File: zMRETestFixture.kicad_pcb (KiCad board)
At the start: 2 copper layers, 106.7 x 124.5 mm, 117 parts, among them J1 Conn_01x01, J2 Conn_01x01, J3 Conn_01x01, J4 Conn_01x01, J5 Conn_01x01, J6 Conn_01x01, J7 Conn_02x05_Counter_Clockwise, J8 Conn_01x01_Female, J9 Conn_01x01_Female, SW1 SW_Push, SW2 SW_Push, U1 molex_48pin_MRE

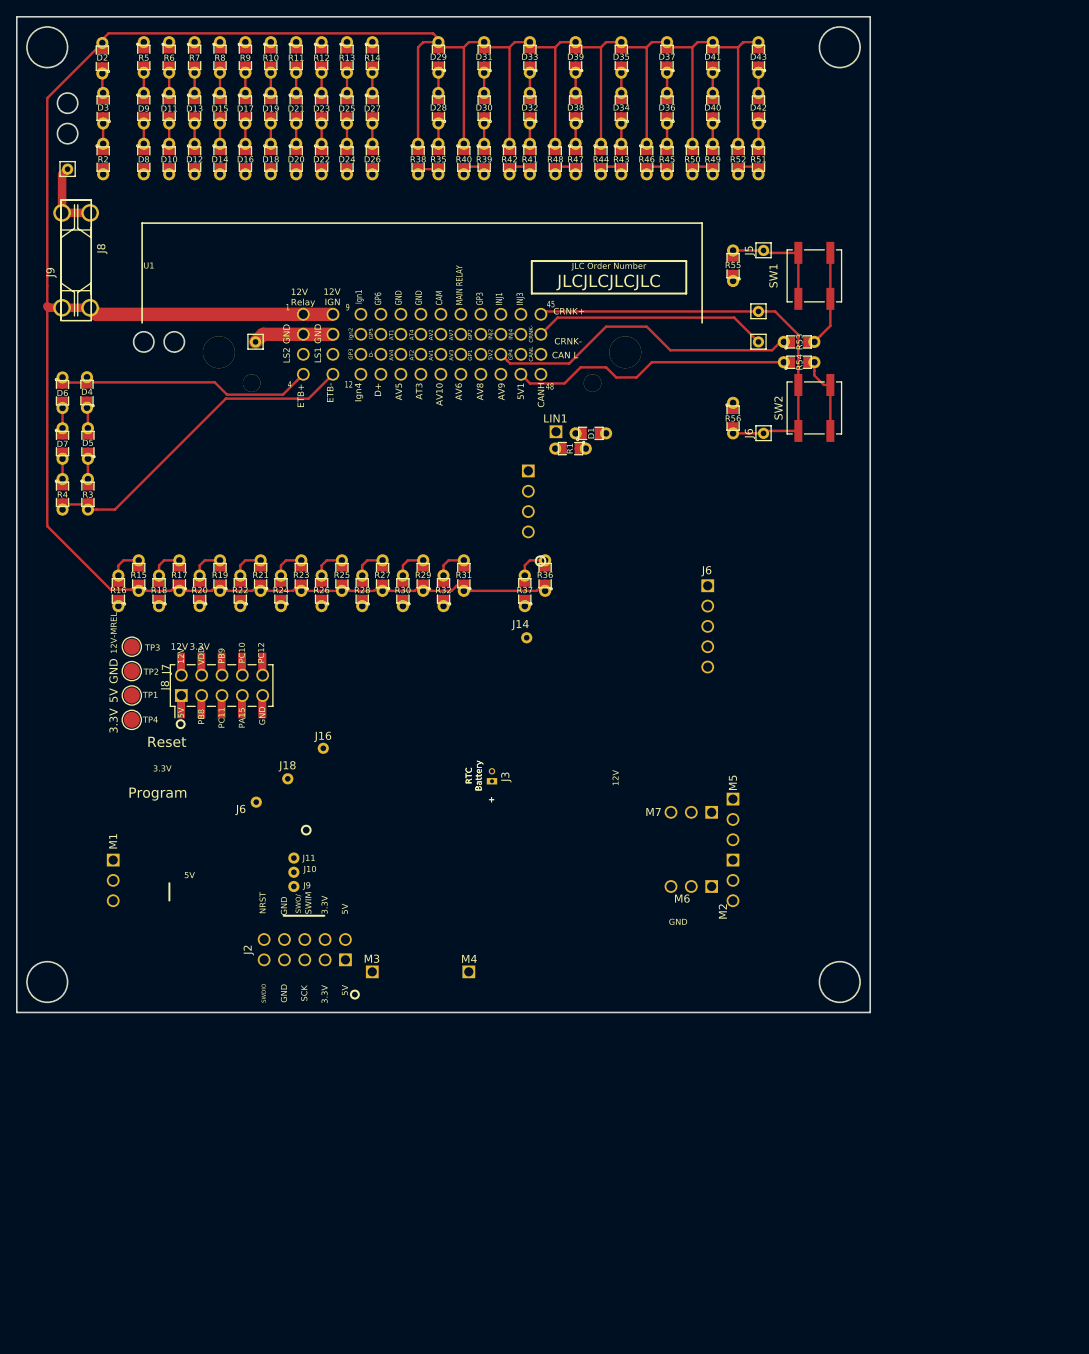
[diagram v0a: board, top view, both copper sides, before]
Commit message: Draft
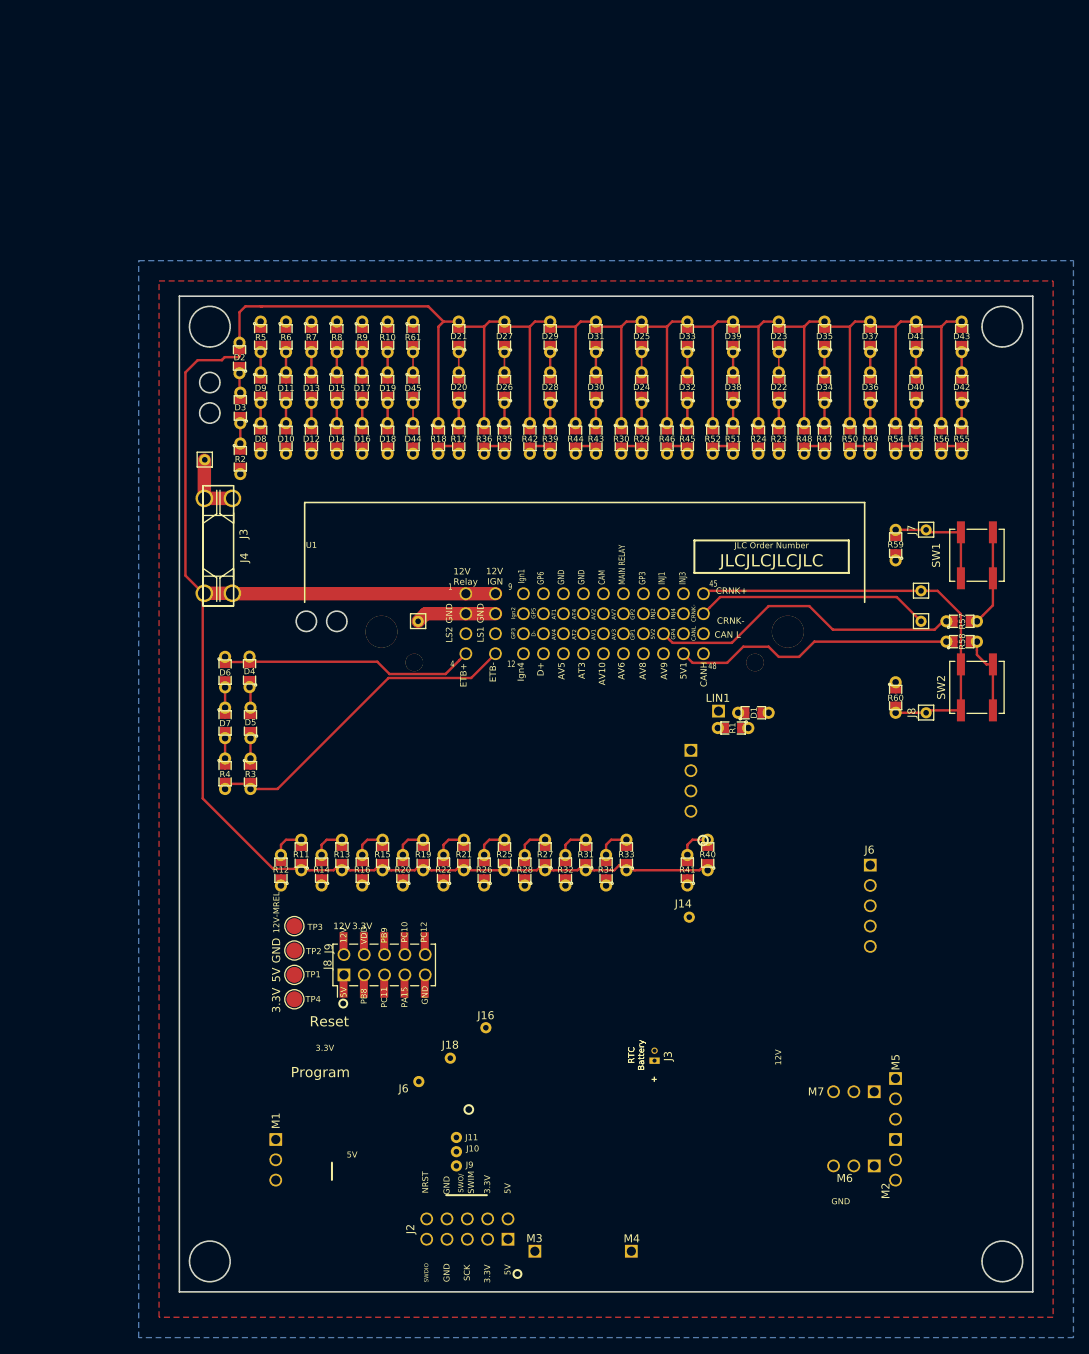
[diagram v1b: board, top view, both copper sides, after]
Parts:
- removed the R11 at (45.1, -2.54)
- removed the R12 at (48.3, -2.54)
- removed the R13 at (51.4, -2.54)
- removed the R14 at (54.6, -2.54)
- removed the R43 at (85.7, 10.2)
- removed the R44 at (83.2, 10.2)
- removed the R45 at (91.4, 10.2)
- removed the R46 at (88.9, 10.2)
- removed the R51 at (102.9, 10.2)
- removed the R52 at (100.3, 10.2)
- added D44: 1N4148WS, rusefi_lib:SM0805_jumper, F.Cu at (59.7, 45.1)
- added D45: GRN, rusefi_lib:SM0805_jumper, F.Cu at (59.7, 38.7)
- added R17: 1k, rusefi_lib:SM0805_jumper, F.Cu at (65.4, 45.1)
- added R18: 5k, rusefi_lib:SM0805_jumper, F.Cu at (62.9, 45.1)
- added R23: 1k, rusefi_lib:SM0805_jumper, F.Cu at (105.4, 45.1)
- added R24: 5k, rusefi_lib:SM0805_jumper, F.Cu at (102.9, 45.1)
- added R29: 1k, rusefi_lib:SM0805_jumper, F.Cu at (88.3, 45.1)
- added R30: 5k, rusefi_lib:SM0805_jumper, F.Cu at (85.7, 45.1)
- added R35: 1k, rusefi_lib:SM0805_jumper, F.Cu at (71.1, 45.1)
- added R36: 5k, rusefi_lib:SM0805_jumper, F.Cu at (68.6, 45.1)
- added R47: 1k, rusefi_lib:SM0805_jumper, F.Cu at (111.1, 45.1)
- added R48: 5k, rusefi_lib:SM0805_jumper, F.Cu at (108.6, 45.1)
- added R53: 1k, rusefi_lib:SM0805_jumper, F.Cu at (122.6, 45.1)
- added R54: 5k, rusefi_lib:SM0805_jumper, F.Cu at (120.0, 45.1)
- added R55: 1k, rusefi_lib:SM0805_jumper, F.Cu at (128.3, 45.1)
- added R56: 5k, rusefi_lib:SM0805_jumper, F.Cu at (125.7, 45.1)
- added R61: 1k, rusefi_lib:SM0805_jumper, F.Cu at (59.7, 32.4)
- D20, D22, D24, D26: value 1N4148WS -> RED
- D21, D23, D25, D27: value BLU -> 1N4148WS
- moved D22 63.9 mm to (105.4, 38.7), turned to 90 degrees
- moved D23 63.9 mm to (105.4, 32.4), turned to 90 degrees
- moved D24 46.6 mm to (88.3, 38.7), turned to 90 degrees
- moved D25 46.6 mm to (88.3, 32.4), turned to 90 degrees
- moved D34 43.2 mm to (111.1, 38.7)
- moved D35 43.2 mm to (111.1, 32.4)
- moved D36 43.2 mm to (116.8, 38.7)
- moved D37 43.2 mm to (116.8, 32.4)
- moved D40 43.2 mm to (122.6, 38.7)
- moved D41 43.2 mm to (122.6, 32.4)
- moved D42 43.2 mm to (128.3, 38.7)
- moved D43 43.2 mm to (128.3, 32.4)
- moved R2 41.2 mm to (38.1, 47.6)
- moved D2 41.2 mm to (38.0, 35.0)
- moved D3 41.2 mm to (38.1, 41.3)
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- renumbered J8 to J3, J9 to J4, J3 to J5, J4 to J6, J5 to J7, J6 to J8, J7 to J9, R15 to R11, R16 to R12, R17 to R13, R18 to R14, R19 to R15, R20 to R16, R21 to R19, R22 to R20, R23 to R21, R24 to R22, R29 to R31, R30 to R32, R31 to R33, R32 to R34, R35 to R39, R36 to R40, R37 to R41, R38 to R42, R39 to R43, R40 to R44, R41 to R45, R42 to R46, R47 to R51, R48 to R52, R53 to R57, R54 to R58, R55 to R59, R56 to R60
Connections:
- D16 pad 2: /GP1 -> /GP6
- D18 pad 2: /GP2 -> /GP5
- D20 pad 2: /GP3 -> Net-(D20-Pad2)
- D21 pad 1: Net-(D21-Pad1) -> Net-(D20-Pad2)
- D21 pad 2: Net-(D20-Pad1) -> /12V_KEY
- D22 pad 2: /GP4 -> Net-(D22-Pad2)
- D23 pad 1: Net-(D23-Pad1) -> Net-(D22-Pad2)
- D23 pad 2: Net-(D22-Pad1) -> /12V_KEY
- D24 pad 2: /GP5 -> Net-(D24-Pad2)
- D25 pad 1: Net-(D25-Pad1) -> Net-(D24-Pad2)
- D25 pad 2: Net-(D24-Pad1) -> /12V_KEY
- D26 pad 2: /GP6 -> Net-(D26-Pad2)
- D27 pad 1: Net-(D27-Pad1) -> Net-(D26-Pad2)
- D27 pad 2: Net-(D26-Pad1) -> /12V_KEY
- R39 pad 2: /AV10 -> /GP2
- R42 pad 2: /AV10 -> /GP2
- R43 pad 2: /AV6 -> /GP1
- R44 pad 2: /AV6 -> /GP1
- R49 pad 1: Net-(D40-Pad1) -> Net-(D36-Pad1)
- R49 pad 2: /INJECTOR-3 -> /INJECTOR-2
- R50 pad 2: /INJECTOR-3 -> /INJECTOR-2
- U1 pad 13: (no net) -> /GP6
- U1 pad 14: (no net) -> /GP5
- U1 pad 29: (no net) -> /MAIN_RELAY
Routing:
- net /12V_KEY: track 358.2 -> 421.9 mm
- net Net-(D44-Pad1): track 0.00 -> 3.81 mm
- net Net-(D26-Pad2): track 0.00 -> 3.18 mm
- net Net-(D22-Pad2): track 0.00 -> 3.18 mm
- net Net-(D20-Pad2): track 0.00 -> 3.18 mm
- net Net-(D27-Pad1): track 3.17 -> 0.00 mm
- net Net-(D25-Pad1): track 3.17 -> 0.00 mm
- net Net-(D23-Pad1): track 3.17 -> 0.00 mm
- net Net-(D21-Pad1): track 3.17 -> 0.00 mm
- net Net-(D45-Pad1): track 0.00 -> 3.17 mm
- net Net-(D24-Pad2): track 0.00 -> 3.17 mm
- net /AV10: track 2.80 -> 0.00 mm
- net /GP3: track 0.00 -> 2.54 mm
- net /GP4: track 0.00 -> 2.54 mm
- net /GP2: track 0.00 -> 2.54 mm
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- added copper zone on B.Cu, net GND
- added copper zone on F.Cu, net GND
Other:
- outline, holes or cut-outs redrawn
